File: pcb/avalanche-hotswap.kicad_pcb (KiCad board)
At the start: 2 copper layers, 179.7 x 122.7 mm, 138 parts, among them J1 TRRS, J2 OLED, P1 i2c_pin, P2 i2c_pin, P3 battery+, P4 battery-, SW0 SW_Push, SW1 SW_Push, SW10 SW_Push, SW11 SW_Push, SW12 SW_Push, SW13 SW_Push, SW14 SW_Push, SW15 SW_Push, SW16 SW_Push, SW17 SW_Push, SW18 SW_Push, SW19 SW_Push, SW2 SW_Push, SW20 SW_Push, SW21 SW_Push, SW22 SW_Push, SW23 SW_Push, SW24 SW_Push, SW25 SW_Push, SW26 SW_Push, SW27 SW_Push, SW28 SW_Push, SW29 SW_Push, SW3 SW_Push, SW30 SW_Push, SW31 SW_Push, SW32 SW_Push, SW33 SW_DPDT_x2, SW34 SW_DPDT_x2, SW4 SW_Push, SW5 SW_Push, SW6 SW_Push, SW7 SW_Push, SW8 SW_Push, SW9 SW_Push, U1 ProMicro

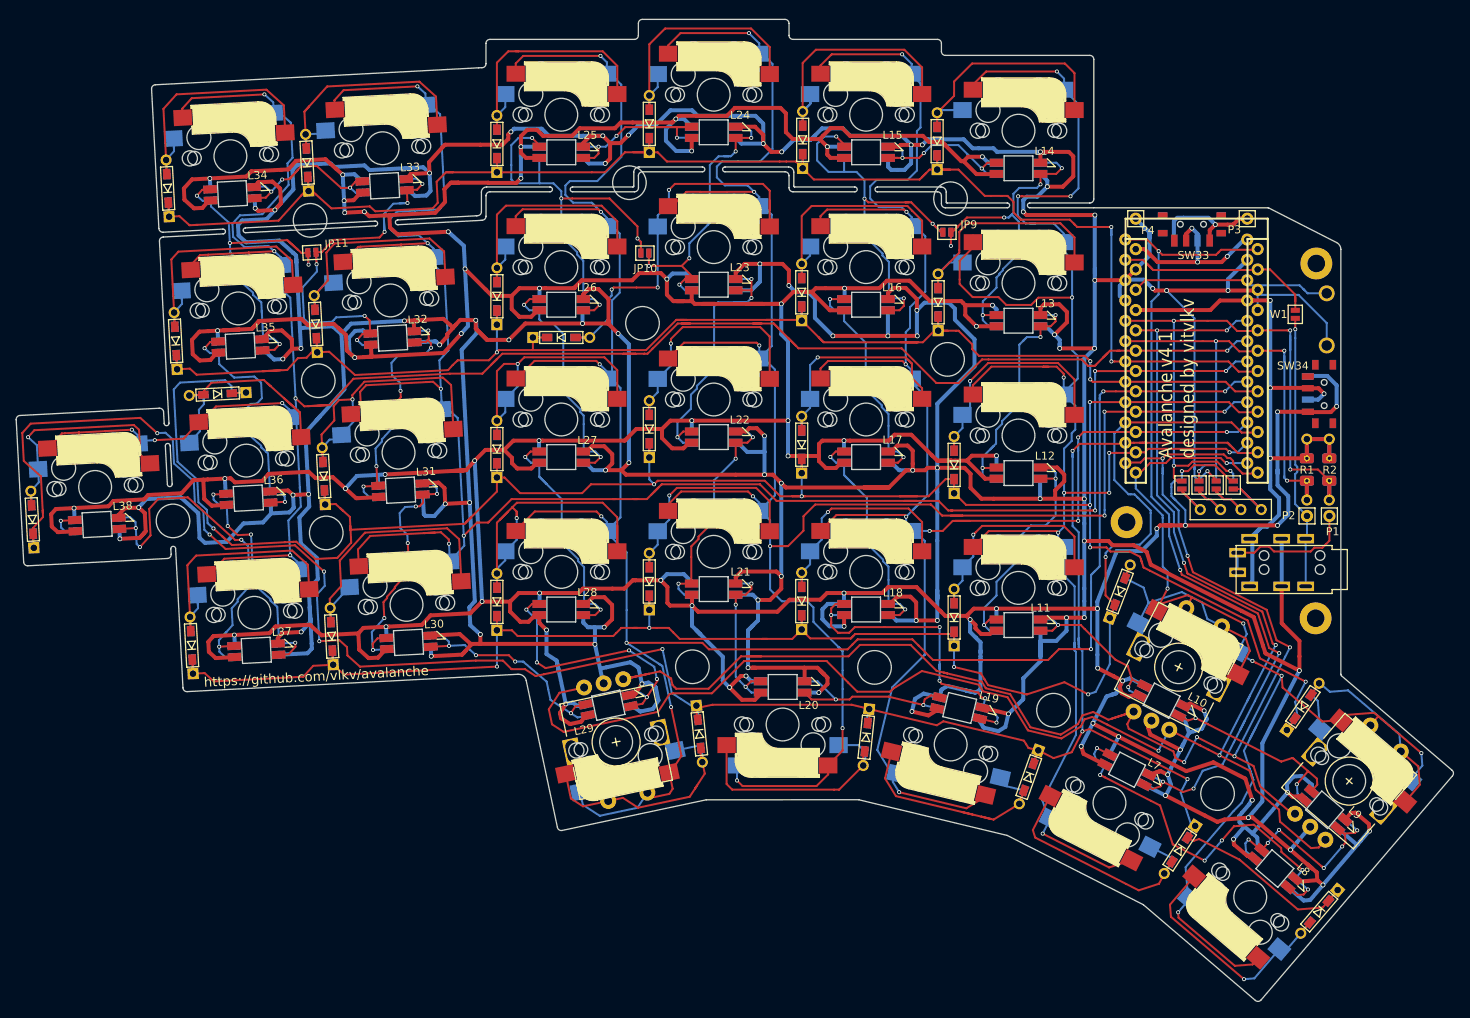
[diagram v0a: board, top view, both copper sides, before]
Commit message: Avalanche with palm key.
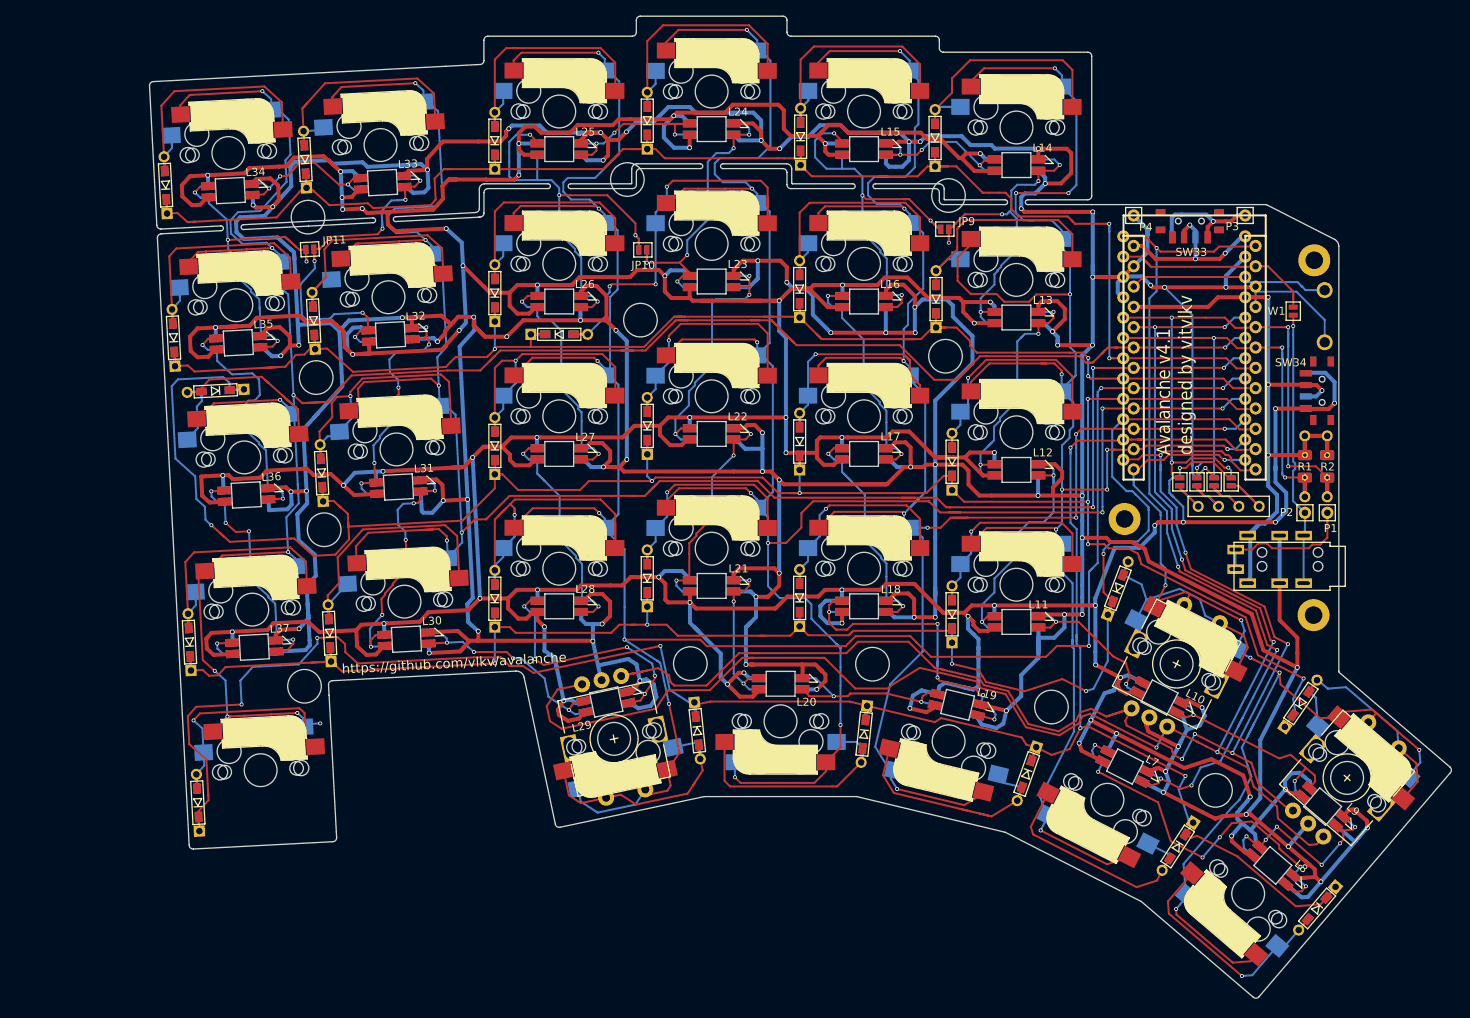
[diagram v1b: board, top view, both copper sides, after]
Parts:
- removed L38: SK6812MINI_LED, used_footprints:YS-SK6812MINI-E
- moved D27 41.0 mm to (83.4, 124.3)
- moved SW27 41.0 mm to (91.3, 120.3)
- moved HM5 26.4 mm to (96.8, 109.8)
- moved D28 0.47 mm to (145.9, 115.3)
- moved SW16 0.47 mm to (147.7, 73.5)
- moved SW30 0.47 mm to (177.3, 116.7)
- moved SW33 0.47 mm to (207.4, 51.6)
- moved D7 0.47 mm to (80.4, 66.2)
- moved L35 0.47 mm to (88.5, 66.8)
- moved JP1 0.47 mm to (206.2, 84.2)
- moved L10 0.47 mm to (203.6, 111.2)
- moved SW29 0.47 mm to (156.3, 114.2)
- moved SW2 0.47 mm to (106.3, 42.1)
- moved D10 0.47 mm to (128.6, 65.8)
- moved D13 0.47 mm to (85.7, 72.9)
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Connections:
- D27 pad 2: Net-(D27-Pad2) -> (no net)
- SW27 pad 1: Net-(D27-Pad2) -> (no net)
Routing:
- net Net-(L37-Pad2): track 47.7 -> 4.68 mm, vias 4 -> 1
- net row4: track 309.6 -> 272.6 mm, vias 8 -> 6
- net GND: track 1149.7 -> 1115.2 mm, vias 77 -> 75
- net (no net): track 0.09 -> 30.5 mm, vias 0 -> 1
- net Net-(D27-Pad2): track 30.4 -> 0.00 mm, vias 1 -> 0
- net VCC: track 973.6 -> 946.7 mm, vias 63 -> 62
- net col0: track 286.7 -> 300.1 mm, vias 8 -> 10
- net Net-(L38-Pad2): track 4.60 -> 0.00 mm, vias 1 -> 0
- net row3: track 215.0 -> 217.2 mm
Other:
- board size 179.7 x 122.7 mm -> 162.7 x 122.7 mm
